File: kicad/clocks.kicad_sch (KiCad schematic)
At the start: 38 parts, among them U1 SIT5156A, U2 ICE40LP384-SG32, U3 LMK1C1104, U4 LEA-M8T, U5 TDC7200, U6 LMK1C1104

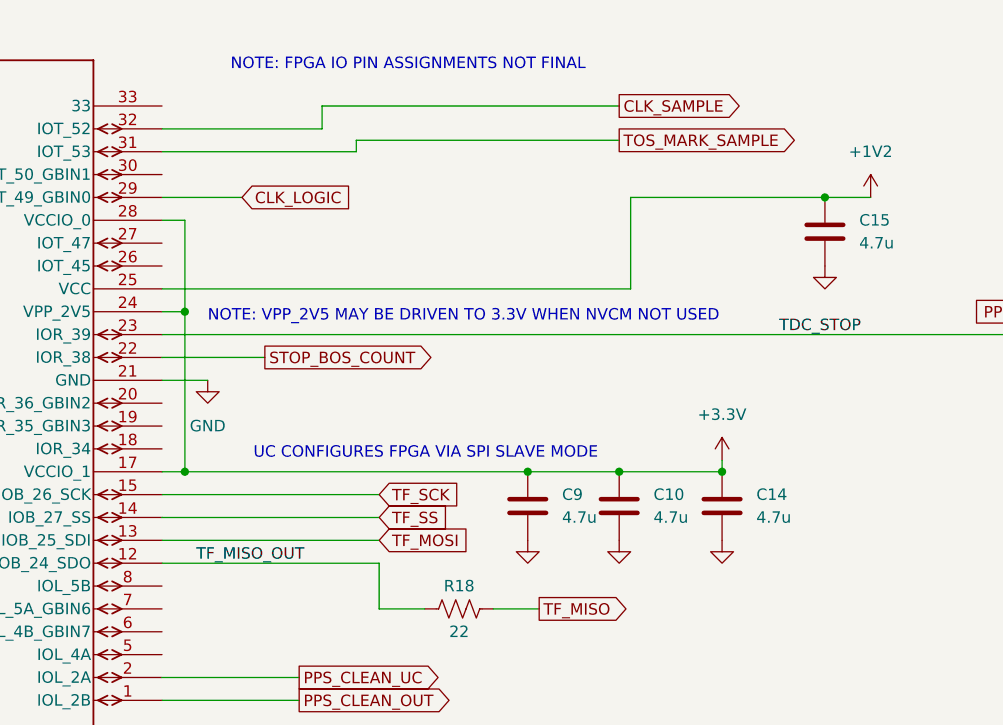
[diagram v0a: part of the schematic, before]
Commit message: updates
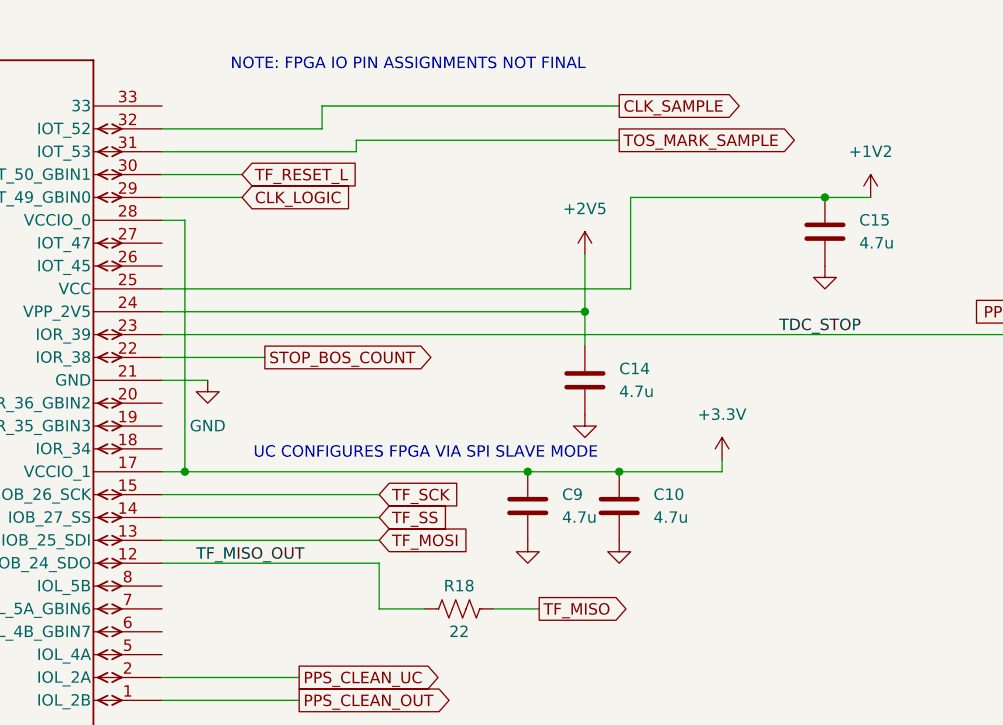
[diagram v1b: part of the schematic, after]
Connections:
- net +3.3V: no longer C14.1, U2.24 (VPP_2V5)
- net TF_RESET_L: now reaches U2.30 (IOT_50_GBIN1)
- new net +2V5: C14.1, U2.24 (VPP_2V5)
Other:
- note removed: "NOTE: VPP_2V5 MAY BE DRIVEN TO 3.3V WHEN NVCM NOT USED"
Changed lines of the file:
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@@
   (junction (at 256.54 60.96) (diameter 0) (color 0 0 0 0)
   )
-  (junction (at 172.72 201.93) (diameter 0) (color 0 0 0 0)
-  )
   (junction (at 135.89 36.83) (diameter 0) (color 0 0 0 0)
   )
   (junction (at 172.72 219.71) (diameter 0) (color 0 0 0 0)
   )
-  (junction (at 232.41 219.71) (diameter 0) (color 0 0 0 0)
-  )
   (junction (at 210.82 219.71) (diameter 0) (color 0 0 0 0)
   )
   (junction (at 220.98 219.71) (diameter 0) (color 0 0 0 0)
   )
+  (junction (at 217.17 201.93) (diameter 0) (color 0 0 0 0)
+  )
   (junction (at 69.85 33.02) (diameter 0) (color 0 0 0 0)
   )
@@
     (stroke (width 0) (type default))
   )
+  (wire (pts (xy 170.18 201.93) (xy 217.17 201.93))
+    (stroke (width 0) (type default))
+  )
   (wire (pts (xy 331.47 100.33) (xy 335.28 100.33))
     (stroke (width 0) (type default))
@@
     (stroke (width 0) (type default))
   )
+  (wire (pts (xy 217.17 201.93) (xy 217.17 195.58))
+    (stroke (width 0) (type default))
+  )
   (wire (pts (xy 83.82 181.61) (xy 80.01 181.61))
     (stroke (width 0) (type default))
@@
     (stroke (width 0) (type default))
   )
+  (wire (pts (xy 170.18 186.69) (xy 179.07 186.69))
+    (stroke (width 0) (type default))
+  )
   (wire (pts (xy 290.83 58.42) (xy 290.83 67.31))
     (stroke (width 0) (type default))
@@
     (stroke (width 0) (type default))
   )
-  (wire (pts (xy 170.18 201.93) (xy 172.72 201.93))
-    (stroke (width 0) (type default))
-  )
   (wire (pts (xy 194.31 229.87) (xy 194.31 234.95))
     (stroke (width 0) (type default))
@@
     (stroke (width 0) (type default))
   )
+  (wire (pts (xy 217.17 201.93) (xy 217.17 205.74))
+    (stroke (width 0) (type default))
+  )
   (wire (pts (xy 160.02 55.88) (xy 154.94 55.88))
     (stroke (width 0) (type default))
@@
     (stroke (width 0) (type default))
   )
-  (wire (pts (xy 172.72 201.93) (xy 172.72 219.71))
-    (stroke (width 0) (type default))
-  )
   (wire (pts (xy 172.72 50.8) (xy 176.53 50.8))
     (stroke (width 0) (type default))
@@
     (stroke (width 0) (type default))
   )
-  (wire (pts (xy 172.72 191.77) (xy 172.72 201.93))
+  (wire (pts (xy 172.72 191.77) (xy 172.72 219.71))
     (stroke (width 0) (type default))
   )
@@
   )
   (text "ADD VCTCXO OPTION HERE" (at 96.52 123.19 0)
-    (effects (font (size 1.27 1.27)) (justify left bottom))
-  )
-  (text "NOTE: VPP_2V5 MAY BE DRIVEN TO 3.3V WHEN NVCM NOT USED"
-    (at 175.26 203.2 0)
     (effects (font (size 1.27 1.27)) (justify left bottom))
   )
@@
     (effects (font (size 1.27 1.27)) (justify left))
     (property "Intersheetrefs" "${INTERSHEET_REFS}" (at 358.7666 214.63 0)
+      (effects (font (size 1.27 1.27)) (justify left) hide)
+    )
+  )
+  (global_label "TF_RESET_L" (shape input) (at 179.07 186.69 0) (fields_autoplaced)
+    (effects (font (size 1.27 1.27)) (justify left))
+    (property "Intersheetrefs" "${INTERSHEET_REFS}" (at 192.8198 186.69 0)
       (effects (font (size 1.27 1.27)) (justify left) hide)
     )
@@
         (path "/c3c549bc-9d82-4b6a-bdb9-a3870905229d/70e7e3a4-572d-4c59-9c26-94e3cd20e23c"
           (reference "R11") (unit 1)
-        )
-      )
-    )
-  )
-  (symbol (lib_id "Device:C") (at 232.41 223.52 0) (unit 1)
-    (in_bom yes) (on_board yes) (dnp no) (fields_autoplaced)
-    (property "Reference" "C14" (at 236.22 222.25 0)
-      (effects (font (size 1.27 1.27)) (justify left))
-    )
-    (property "Value" "4.7u" (at 236.22 224.79 0)
-      (effects (font (size 1.27 1.27)) (justify left))
-    )
-    (property "Footprint" "" (at 233.3752 227.33 0)
-      (effects (font (size 1.27 1.27)) hide)
-    )
-    (property "Datasheet" "~" (at 232.41 223.52 0)
-      (effects (font (size 1.27 1.27)) hide)
-    )
-    (pin "1")
-    (pin "2")
-    (instances
-      (project "gpsrx"
-        (path "/c3c549bc-9d82-4b6a-bdb9-a3870905229d/70e7e3a4-572d-4c59-9c26-94e3cd20e23c"
-          (reference "C14") (unit 1)
         )
       )
@@
     )
   )
+  (symbol (lib_id "power:+2V5") (at 217.17 195.58 0) (unit 1)
+    (in_bom yes) (on_board yes) (dnp no) (fields_autoplaced)
+    (property "Reference" "#PWR063" (at 217.17 199.39 0)
+      (effects (font (size 1.27 1.27)) hide)
+    )
+    (property "Value" "+2V5" (at 217.17 190.5 0)
+      (effects (font (size 1.27 1.27)))
+    )
+    (property "Footprint" "" (at 217.17 195.58 0)
+      (effects (font (size 1.27 1.27)) hide)
+    )
+    (property "Datasheet" "" (at 217.17 195.58 0)
+      (effects (font (size 1.27 1.27)) hide)
+    )
+    (pin "1")
+    (instances
+      (project "gpsrx"
+        (path "/c3c549bc-9d82-4b6a-bdb9-a3870905229d/70e7e3a4-572d-4c59-9c26-94e3cd20e23c"
+          (reference "#PWR063") (unit 1)
+        )
+      )
+    )
+  )
   (symbol (lib_id "power:GND") (at 251.46 123.19 0) (unit 1)
     (in_bom yes) (on_board yes) (dnp no) (fields_autoplaced)
@@
     )
   )
-  (symbol (lib_id "power:GND") (at 232.41 227.33 0) (unit 1)
-    (in_bom yes) (on_board yes) (dnp no) (fields_autoplaced)
-    (property "Reference" "#PWR040" (at 232.41 233.68 0)
-      (effects (font (size 1.27 1.27)) hide)
-    )
-    (property "Value" "GND" (at 232.41 232.41 0)
-      (effects (font (size 1.27 1.27)) hide)
-    )
-    (property "Footprint" "" (at 232.41 227.33 0)
-      (effects (font (size 1.27 1.27)) hide)
-    )
-    (property "Datasheet" "" (at 232.41 227.33 0)
+  (symbol (lib_id "power:GND") (at 217.17 213.36 0) (unit 1)
+    (in_bom yes) (on_board yes) (dnp no) (fields_autoplaced)
+    (property "Reference" "#PWR040" (at 217.17 219.71 0)
+      (effects (font (size 1.27 1.27)) hide)
+    )
+    (property "Value" "GND" (at 217.17 218.44 0)
+      (effects (font (size 1.27 1.27)) hide)
+    )
+    (property "Footprint" "" (at 217.17 213.36 0)
+      (effects (font (size 1.27 1.27)) hide)
+    )
+    (property "Datasheet" "" (at 217.17 213.36 0)
       (effects (font (size 1.27 1.27)) hide)
     )
@@
         )
       )
+    )
+  )
+  (symbol (lib_id "Device:C") (at 217.17 209.55 0) (unit 1)
+    (in_bom yes) (on_board yes) (dnp no) (fields_autoplaced)
+    (property "Reference" "C14" (at 220.98 208.28 0)
+      (effects (font (size 1.27 1.27)) (justify left))
+    )
+    (property "Value" "4.7u" (at 220.98 210.82 0)
+      (effects (font (size 1.27 1.27)) (justify left))
+    )
+    (property "Footprint" "" (at 218.1352 213.36 0)
+      (effects (font (size 1.27 1.27)) hide)
+    )
+    (property "Datasheet" "~" (at 217.17 209.55 0)
+      (effects (font (size 1.27 1.27)) hide)
+    )
+    (pin "1")
+    (pin "2")
+    (instances
+      (project "gpsrx"
+        (path "/c3c549bc-9d82-4b6a-bdb9-a3870905229d/70e7e3a4-572d-4c59-9c26-94e3cd20e23c"
+          (reference "C14") (unit 1)
+        )
+      )
